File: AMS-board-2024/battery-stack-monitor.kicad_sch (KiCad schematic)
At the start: 52 parts, among them Q115 2N7002K-AU, U15 NV24C16SNVLT3G, U23 LM25180-Q1, U24 LTC2949, U25 NCV8711BMTW500TBG

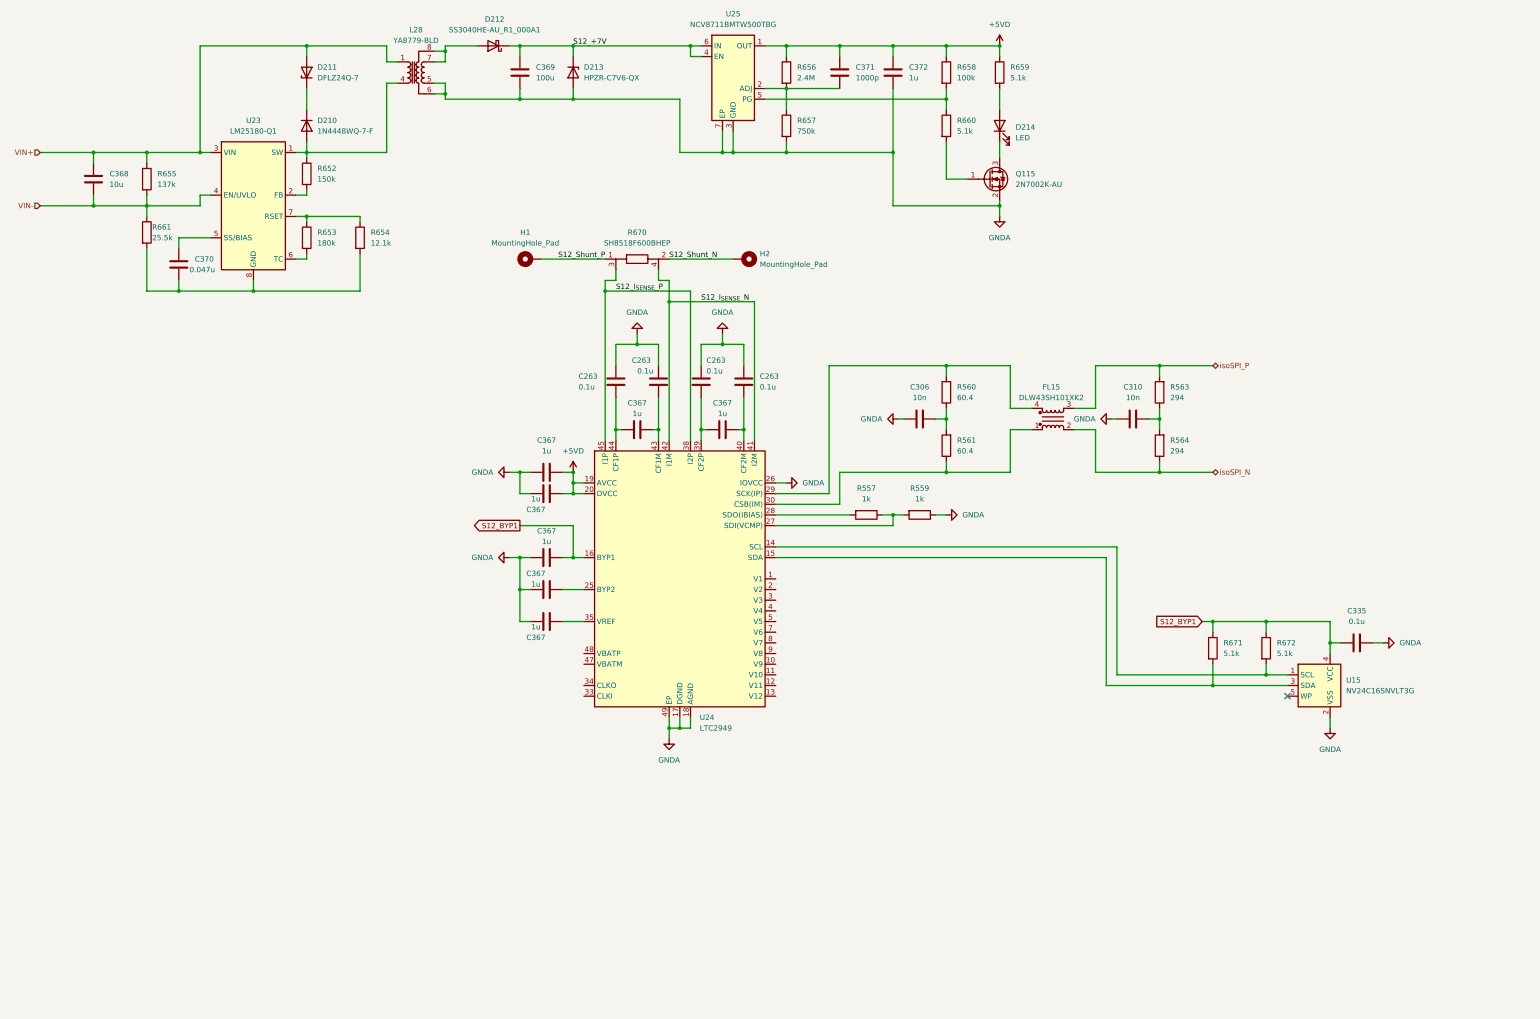
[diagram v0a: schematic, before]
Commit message: Battery Stack Monitor完成
チェック未済
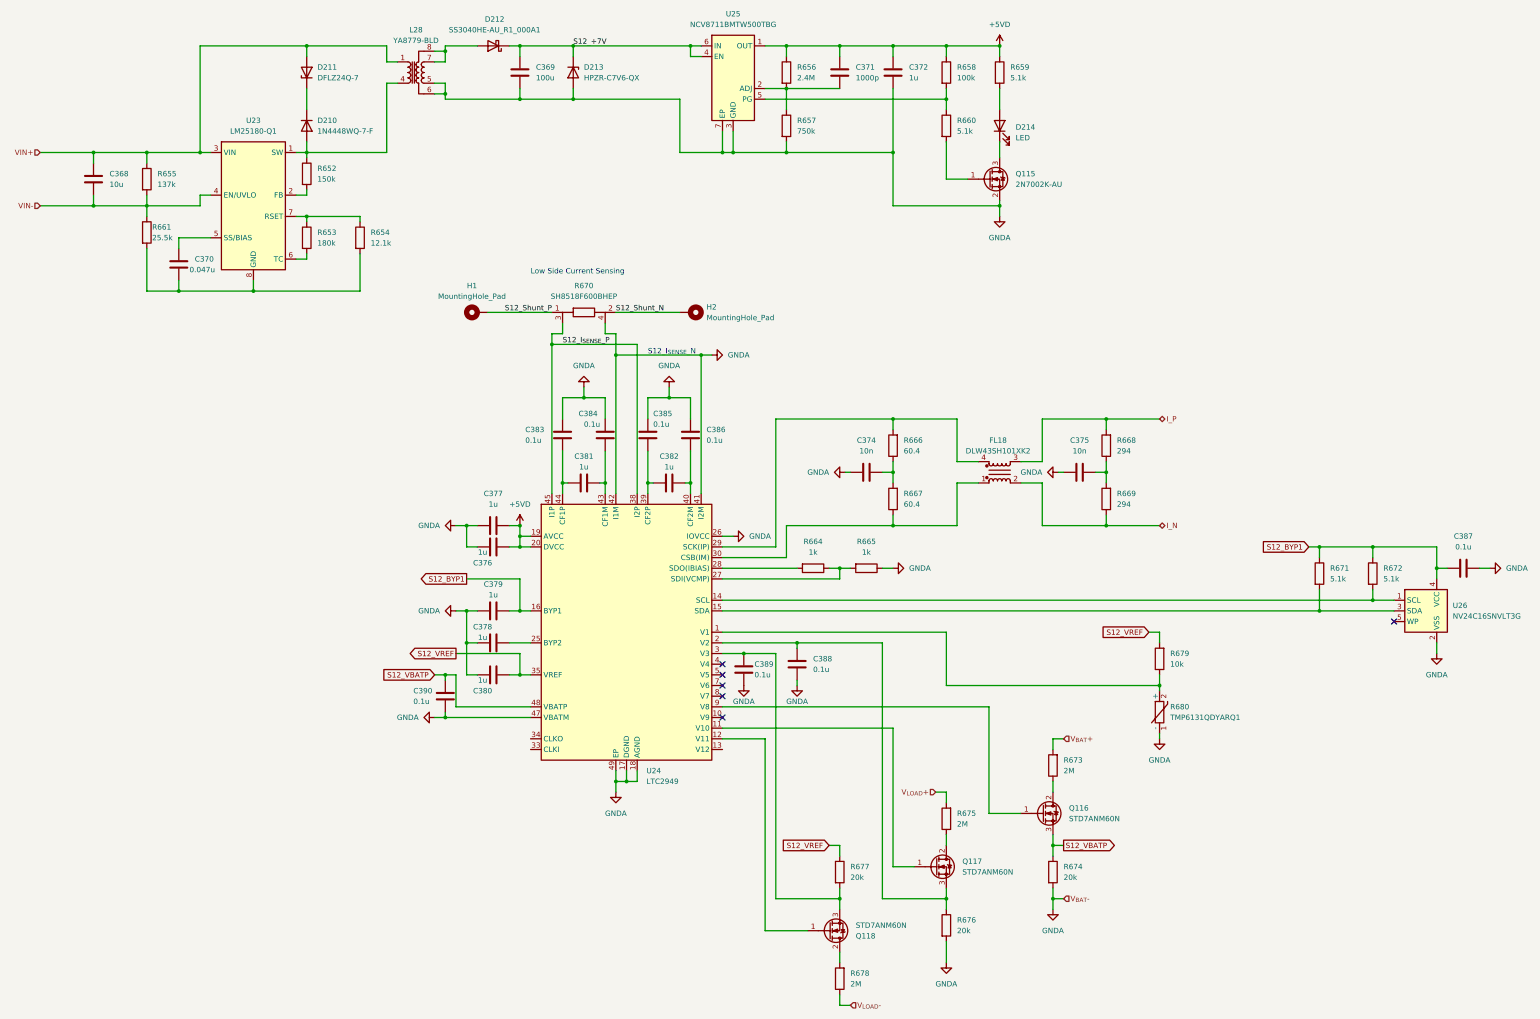
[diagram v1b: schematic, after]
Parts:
- added C388, C389, C390: 0.1u, Capacitor_SMD:C_0603_1608Metric, symbol Device:C
- added Q116, Q117, Q118: STD7ANM60N, ProjectEV:Package_TO-252_STD7ANM60N, symbol ProjectEV:Transistor_STD7ANM60N
- added R673, R675, R678: 2M, Resistor_SMD:R_0603_1608Metric, symbol Device:R
- added R674, R676, R677: 20k, Resistor_SMD:R_0603_1608Metric, symbol Device:R
- added R679: 10k, Resistor_SMD:R_0603_1608Metric, symbol Device:R
- added R680: TMP6131QDYARQ1, ProjectEV:Package_SOD-523_TMP6131QDYARQ1, symbol ProjectEV:Sensor_TMP6131QDYARQ1
- renumbered C306 to C374, C310 to C375, C367 to C376, C367 to C377, C367 to C378, C367 to C379, C367 to C380, C367 to C381, C367 to C382, C263 to C383, C263 to C384, C263 to C385, C263 to C386, C335 to C387, FL15 to FL18, R557 to R664, R559 to R665, R560 to R666, R561 to R667, R563 to R668, R564 to R669, U15 to U26
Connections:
- net S12_I_{SENSE}_N is gone; now on net GNDA: R670.4, U24.41 (I2M), U24.42 (I1M)
- net GNDA: now also U24.47 (VBATM), C388.2, C389.2, C390.2, R674.2, R676.2, R680.1 (-)
- net at U24.1 (V1): now also R679.1, R680.2 (+)
- net at U24.11 (V10): now also Q117.1 (G)
- net at U24.12 (V11): now also Q118.1 (G)
- net at U24.2 (V2): now also C388.1, Q117.3 (S), R676.1
- net at U24.3 (V3): now also C389.1, Q118.3 (S), R677.2
- net S12_VREF: now reaches C380.1, U24.35 (VREF)
- net S12_VREF: now also R677.1, R679.2
- net S12_VBATP: now reaches U24.48 (VBATP)
- net S12_VBATP: now also C390.1, Q116.3 (S), R674.1
- net at U24.9 (V8): now also Q116.1 (G)
- net isoSPI_N renamed I_N
- net isoSPI_P renamed I_P
- new net: Q118.2 (D), R678.2
- new net: Q117.2 (D), R675.1
- new net: Q116.2 (D), R673.1
- new net V_{BAT}+: R673.2
- new net V_{LOAD}+: R675.2
- new net V_{LOAD}-: R678.1
- no-connect marks 1 -> 6
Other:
- note added: "Low Side Current Sensing"
- note added: "S12_I_{SENSE}_N"
- moved on the sheet: C374, C375, C376, C377, C378, C379, C380, C381, C382, C383, C384, C385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
